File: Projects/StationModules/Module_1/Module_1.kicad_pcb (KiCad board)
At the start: 2 copper layers, 166 x 100 mm, 123 parts, among them J2 +310, J3 -310, J4 PowerTrans1, J5 PowerTrans2, M1 BluePillStm32, Q1 STD20NF06T4, Q2 STD20NF06T4, Q3 STD20NF06T4, Q4 STD20NF06T4, Q5 IRGB10B60KD, Q6 IRGB10B60KD, Q7 IRGB10B60KD, Q8 IRGB10B60KD, T1 Transformer_SP_2S, T2 Transformer_SP_2S, U1 PC817, U2 L7805, U3 TC1047AxNB, U5 LM311, U6 6N137

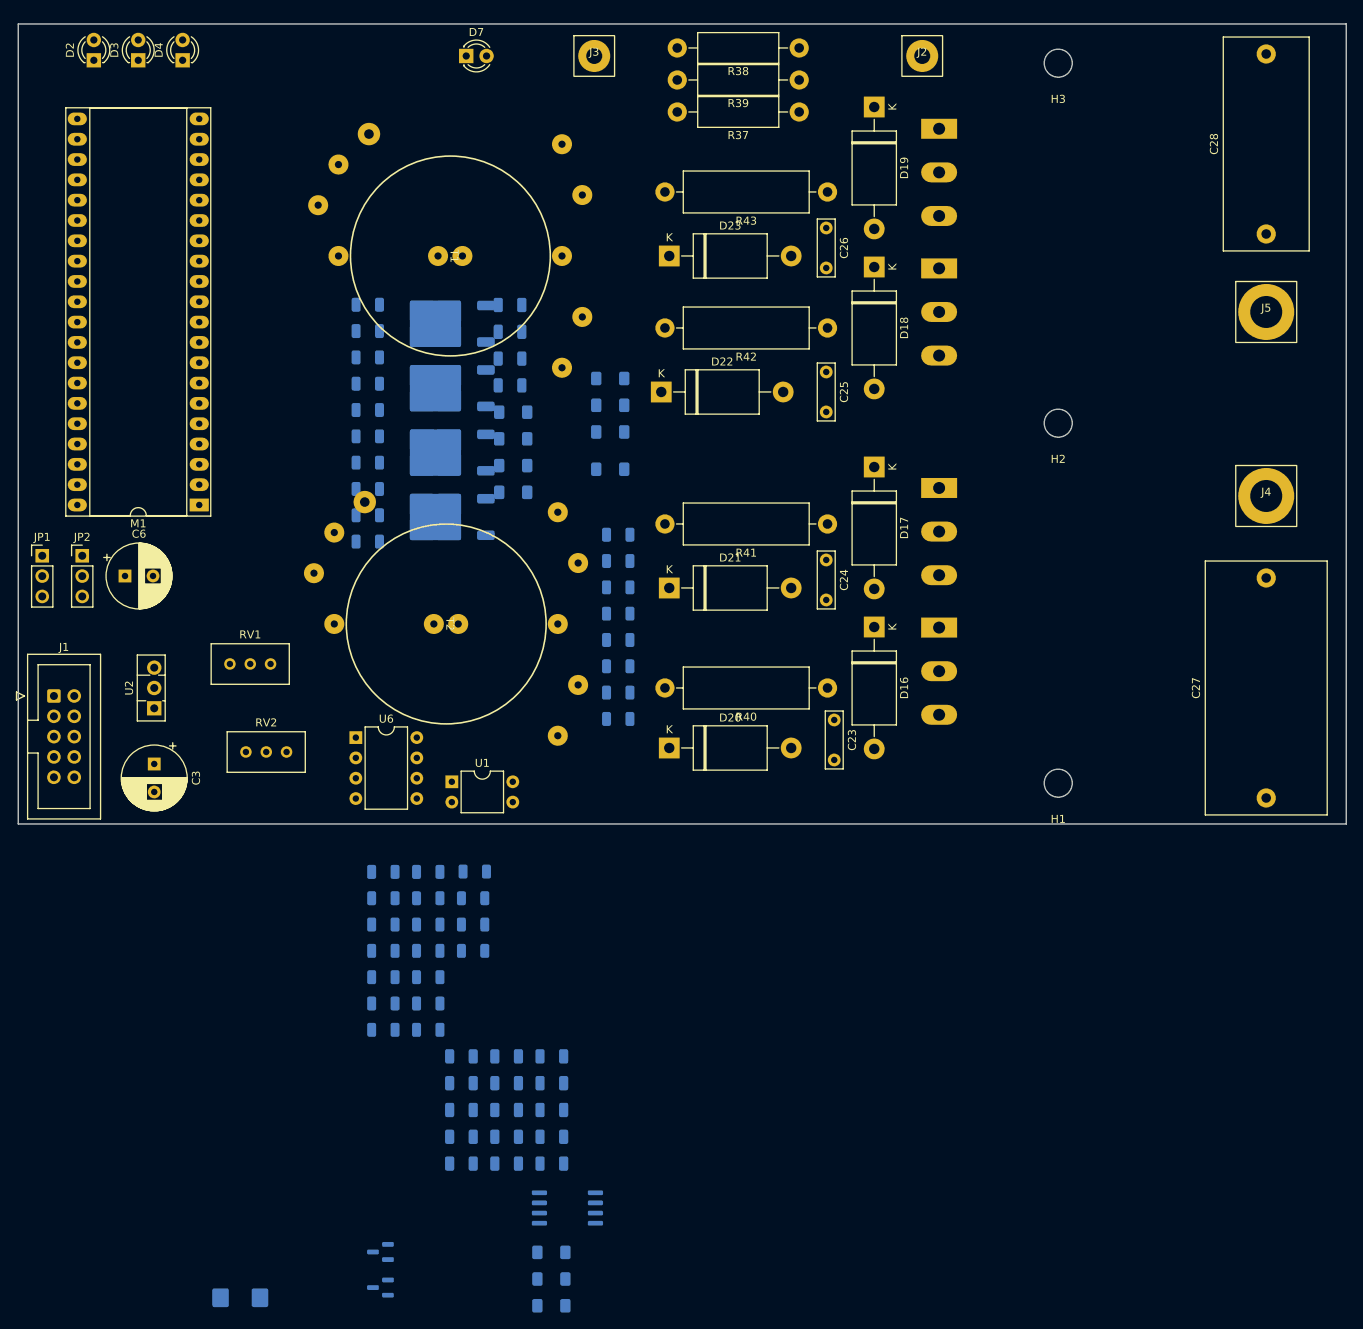
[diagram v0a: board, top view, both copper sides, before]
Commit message: Place elements 2
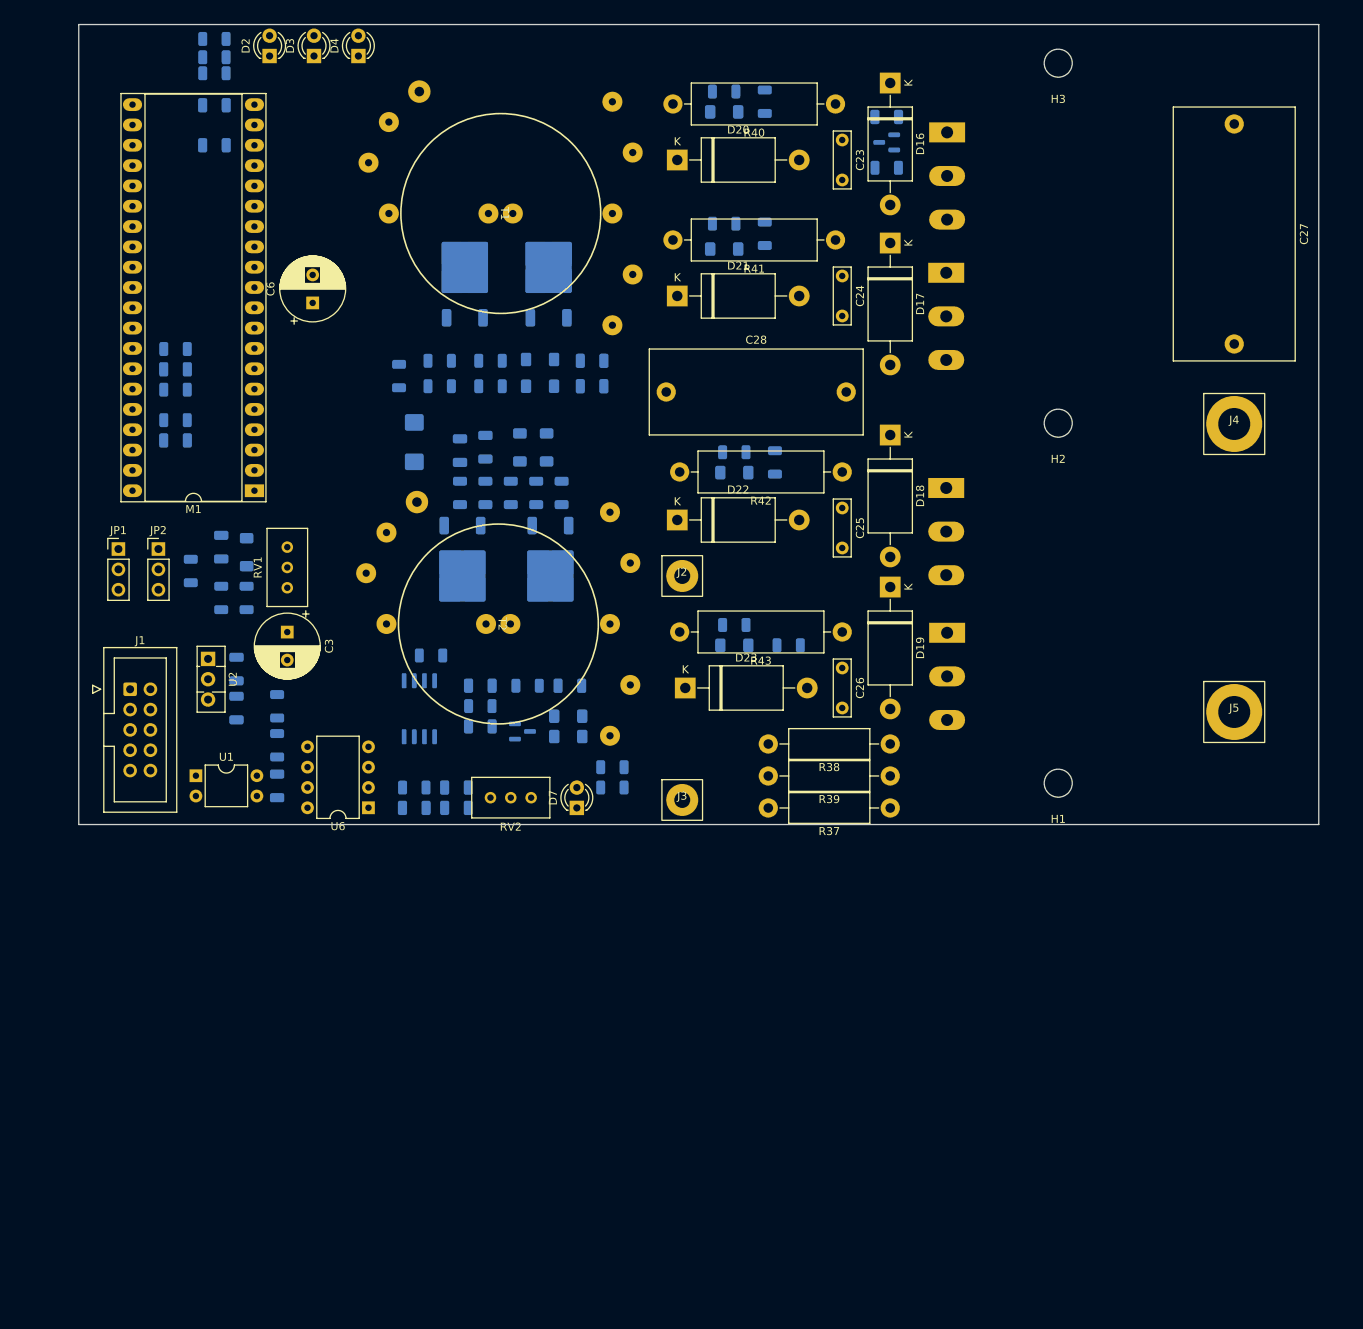
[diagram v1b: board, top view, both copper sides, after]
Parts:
- moved U3 152.5 mm to (162.6, 50.8)
- moved C12 136.0 mm to (162.6, 47.6), turned to 0 degrees
- moved R7 125.6 mm to (78.5, 37.9), turned to 0 degrees
- moved C1 122.8 mm to (78.5, 46.2)
- moved C2 121.2 mm to (78.5, 51.2)
- moved R6 120.1 mm to (78.5, 40.2), turned to 0 degrees
- moved R5 114.9 mm to (78.5, 42.2), turned to 0 degrees
- moved C4 109.1 mm to (103.5, 88.3), turned to 90 degrees
- moved R9 107.8 mm to (162.6, 54.0)
- moved C11 101.4 mm to (73.7, 79.2), turned to 0 degrees
- moved D1 95.4 mm to (82.5, 102.0), turned to -90 degrees
- moved D7 95.0 mm to (123.8, 134.0), turned to 90 degrees
- moved J3 93.6 mm to (137.0, 133.0)
- moved C10 90.4 mm to (73.7, 88.1), turned to 0 degrees
- moved R37 87.7 mm to (163.0, 134.0)
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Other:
- board size 166 x 100 mm -> 155 x 100 mm

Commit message: Trace complit 1
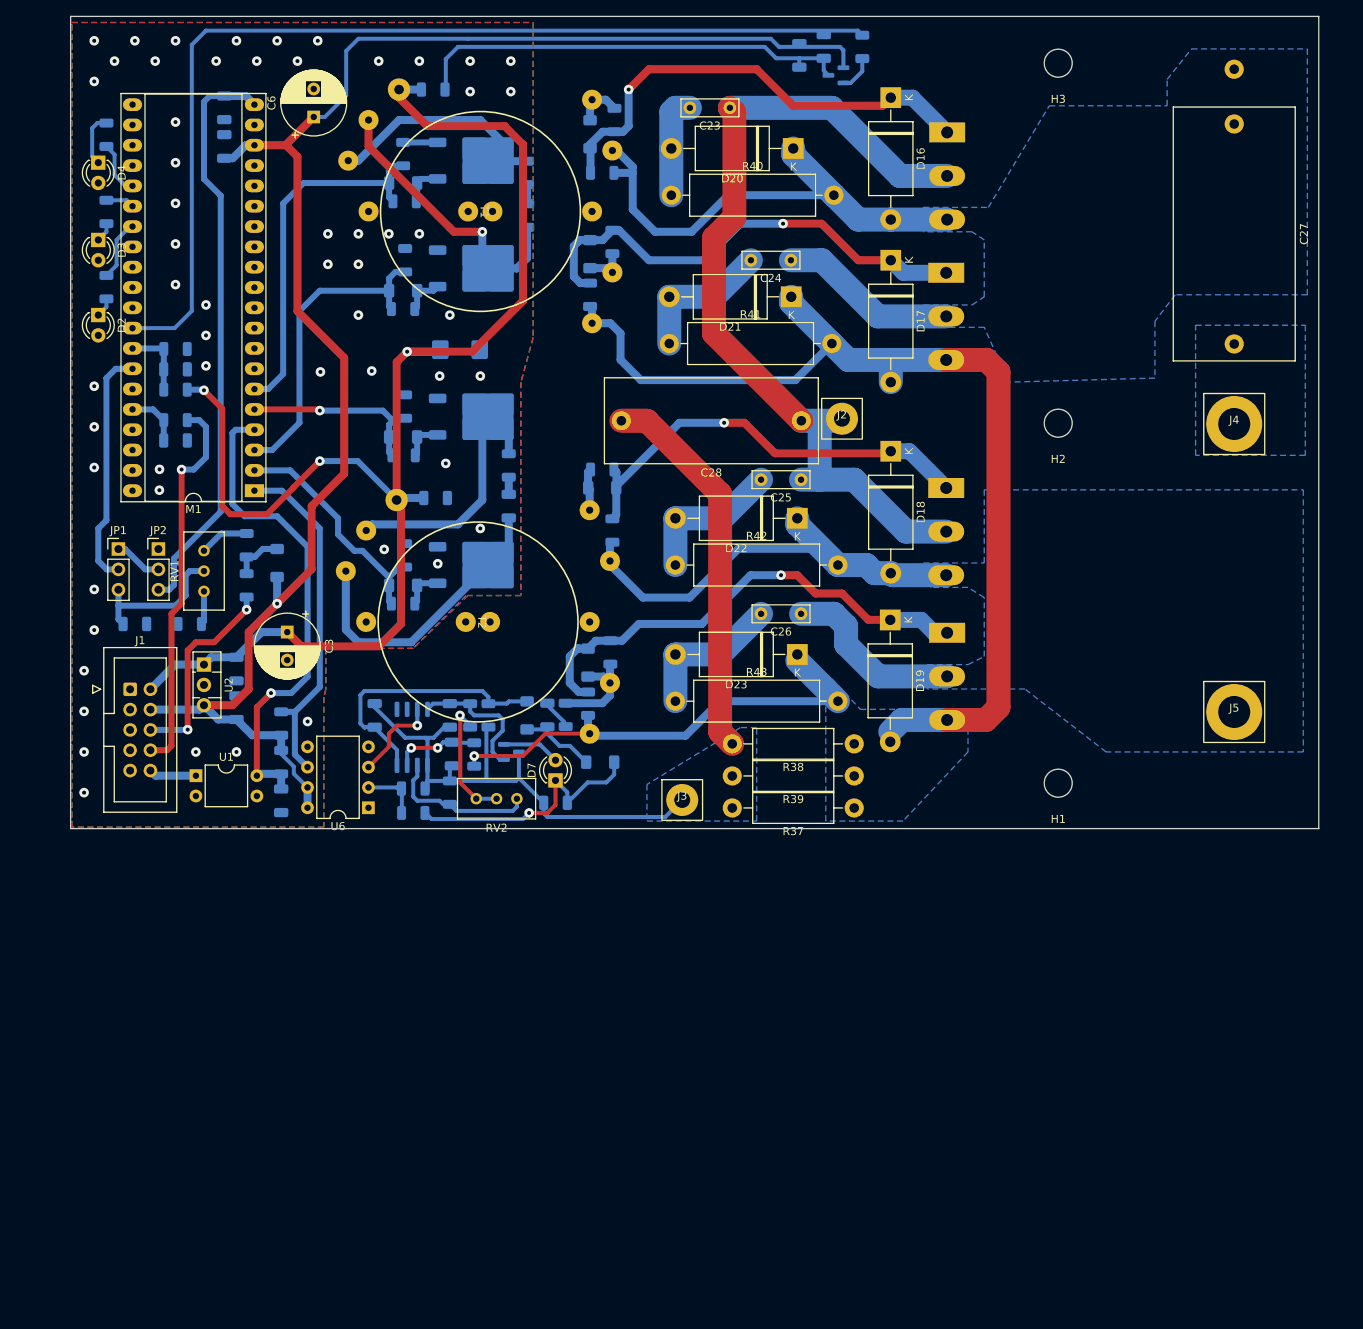
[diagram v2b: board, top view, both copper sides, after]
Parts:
- added ?: , , F.Cu at (206.0, 41.7)
- added C29: 0,1uF, Capacitor_SMD:C_1206_3216Metric, B.Cu at (151.6, 39.9)
- moved C19 42.1 mm to (105.9, 44.2)
- moved D2 38.8 mm to (64.0, 72.4), turned to -90 degrees
- moved D3 35.4 mm to (64.0, 63.0), turned to -90 degrees
- moved D4 35.1 mm to (64.0, 53.3), turned to -90 degrees
- moved R27 30.0 mm to (117.6, 54.6), turned to 90 degrees
- moved R5 30.0 mm to (65.0, 68.9), turned to -90 degrees
- moved J2 28.0 mm to (157.0, 85.3)
- moved D8 27.9 mm to (102.1, 55.9), turned to 0 degrees
- moved R19 26.2 mm to (102.1, 52.3), turned to -90 degrees
- moved R36 26.1 mm to (125.2, 121.0), turned to 90 degrees
- moved R13 25.1 mm to (103.4, 134.6), turned to 180 degrees
- moved D11 24.9 mm to (102.1, 106.2), turned to 0 degrees
- moved R41 24.5 mm to (135.4, 75.9), turned to 0 degrees
- moved R42 23.9 mm to (136.1, 103.6), turned to 0 degrees
- moved R6 23.6 mm to (65.0, 59.5), turned to -90 degrees
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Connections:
- C1 pad 1: +3.3V -> +3V3
- M1 pad 20: +3.3V -> +3V3
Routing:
- net +5V: track 0.00 -> 203.9 mm, vias 0 -> 1
- net /Shunt+: track 0.00 -> 188.1 mm, vias 0 -> 1
- net +12V: track 0.00 -> 181.7 mm, vias 0 -> 3
- net /TMP: track 0.00 -> 126.4 mm
- net /Shunt-: track 0.00 -> 115.0 mm
- net Net-(J2-Pin_1): track 0.00 -> 109.0 mm
- net Net-(D16-A2): track 0.00 -> 85.7 mm
- net Net-(D18-A2): track 0.00 -> 81.3 mm
- net +3V3: track 0.00 -> 72.9 mm
- net /IN_1: track 0.00 -> 61.2 mm, vias 0 -> 1
- net Net-(D13-A): track 0.00 -> 60.4 mm, vias 0 -> 1
- net GND: track 0.00 -> 60.1 mm, vias 0 -> 56
- net Net-(D15-A): track 0.00 -> 59.8 mm, vias 0 -> 1
- net Net-(D14-A): track 0.00 -> 58.9 mm, vias 0 -> 1
- net Net-(D12-A): track 0.00 -> 54.8 mm, vias 0 -> 1
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- added copper zone on B.Cu, net /Shunt+
- added copper zone on B.Cu, net /Shunt-
- added copper zone on B.Cu, net GND
- added copper zone on F.Cu, net GND
- added copper zone on B.Cu, net Net-(D16-A2)
- added copper zone on B.Cu, net Net-(D18-A2)
- added copper zone on B.Cu, net Net-(J4-Pin_1)
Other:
- board size 155 x 100 mm -> 156 x 101.5 mm
